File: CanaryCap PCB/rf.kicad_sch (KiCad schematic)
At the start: 8 parts

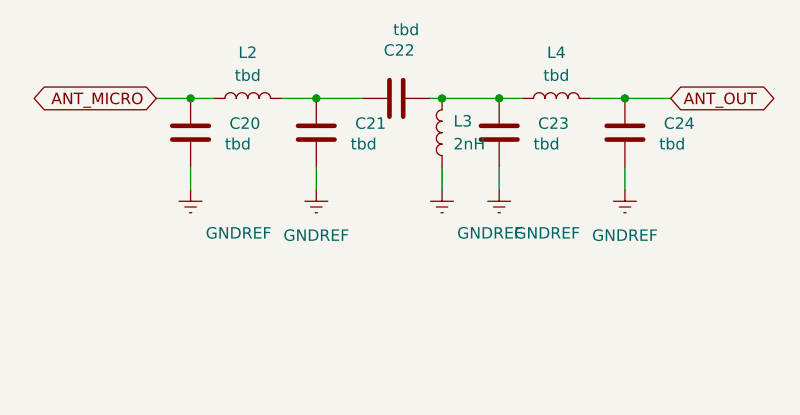
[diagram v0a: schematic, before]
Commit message: Finished level for packaging
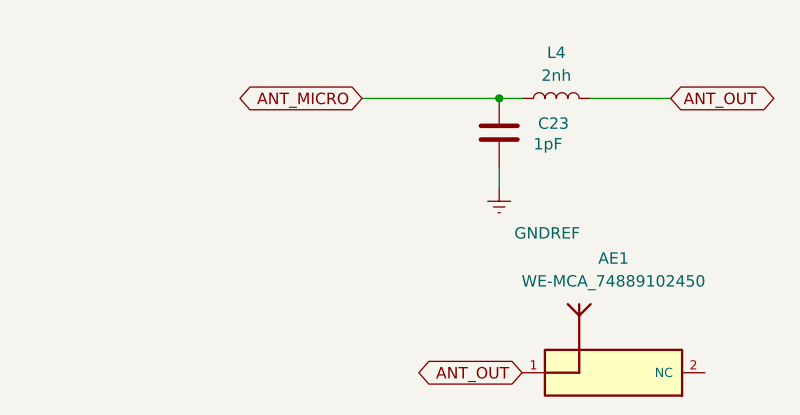
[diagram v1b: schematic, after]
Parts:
- removed C20, C21, C22, C24: tbd, Capacitor_SMD:C_0603_1608Metric_Pad1.08x0.95mm_HandSolder, symbol Device:C
- removed L2: tbd, Inductor_SMD:L_0603_1608Metric, symbol Device:L
- removed L3: 2nH, Inductor_SMD:L_0603_1608Metric, symbol Device:L
- added AE1: WE-MCA_74889102450, Library:WE-MCA_74889102450, symbol ESP-32-C6:WE-MCA_74889102450
- C23: value tbd -> 1pF
- L4: value tbd -> 2nh
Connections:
- net ANT_MICRO: now also C23.1, L4.1
- net ANT_OUT: now also AE1.1
